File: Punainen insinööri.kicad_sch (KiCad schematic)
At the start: 28 parts, among them J1 Barrel_Jack_Switch, Q1 MMBF4393LT1G, SW1 SW_DPDT_x2, U1 LF351D

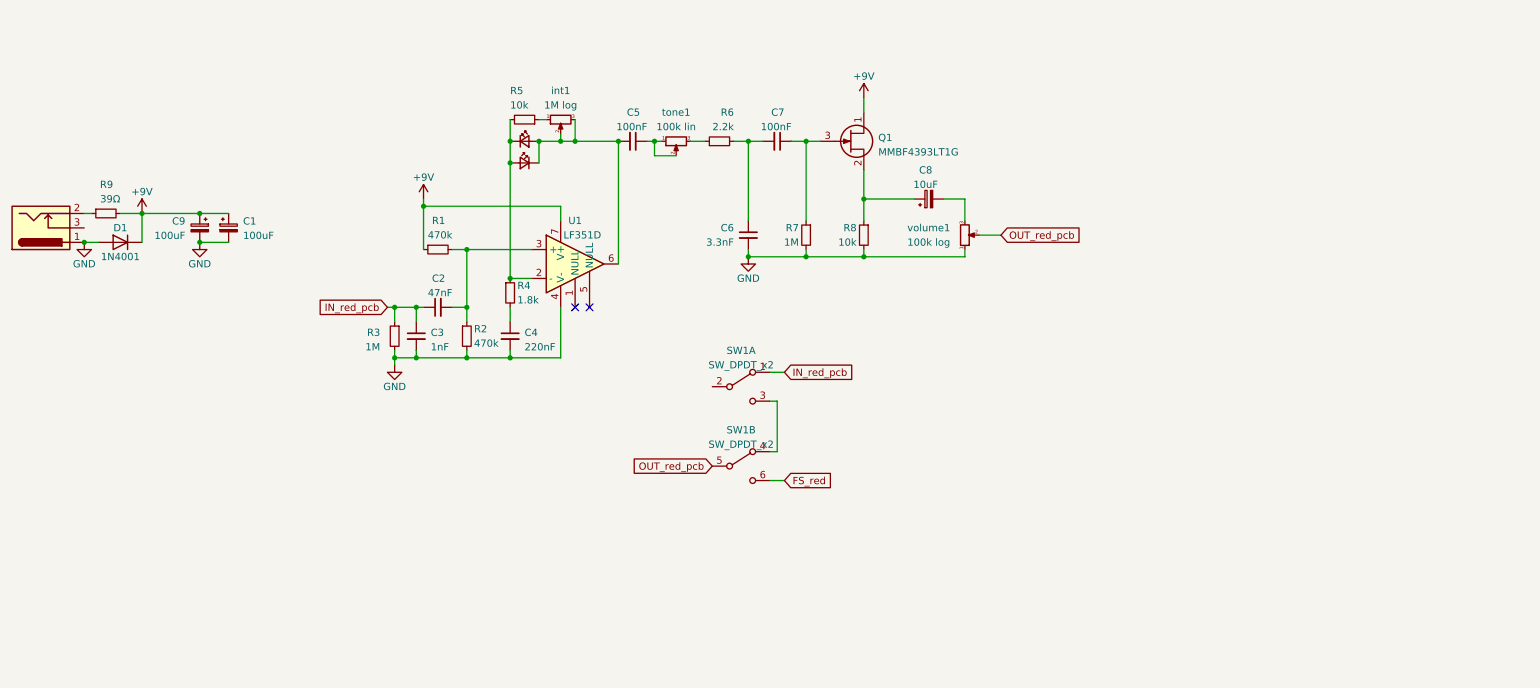
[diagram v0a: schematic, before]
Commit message: small fixes
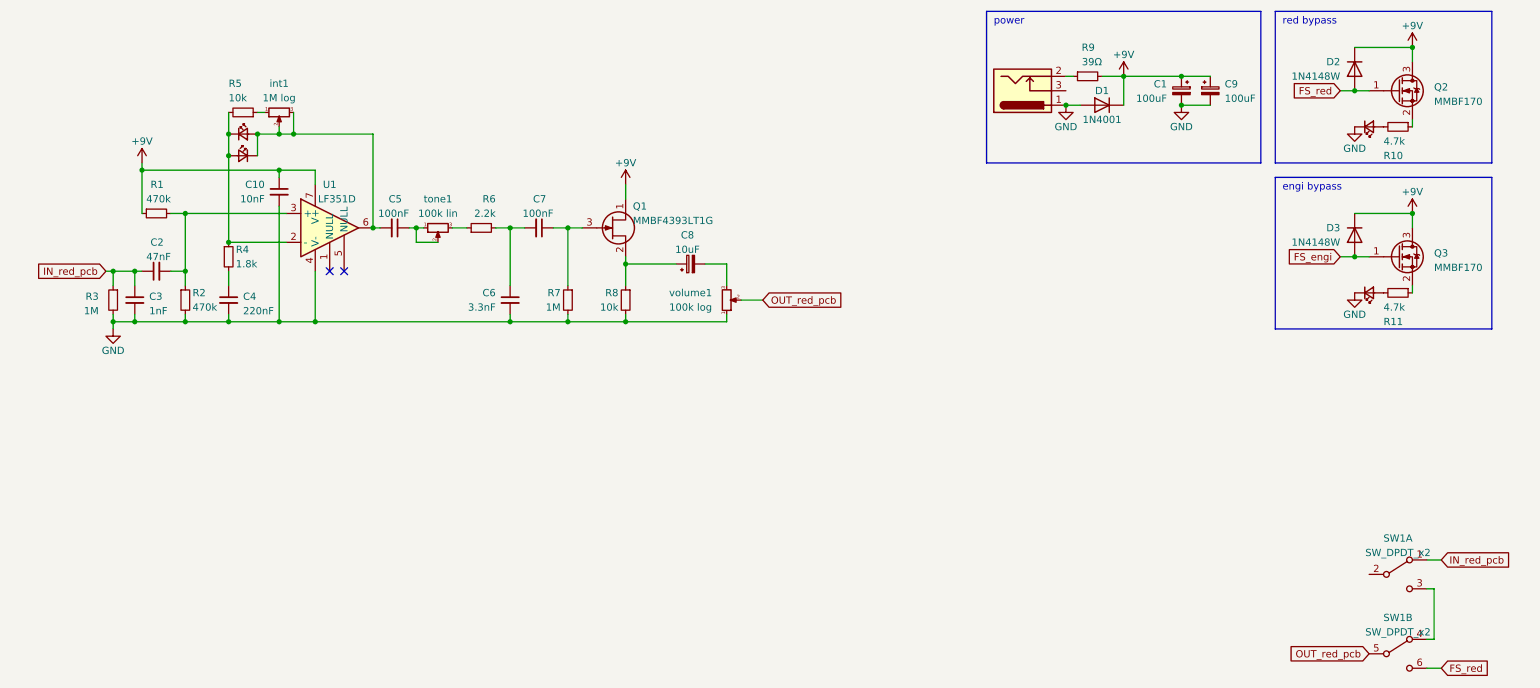
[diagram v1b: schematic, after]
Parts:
- added C10: 10nF, Capacitor_SMD:C_0805_2012Metric_Pad1.18x1.45mm_HandSolder, symbol Device:C_Small
- added D2, D3: 1N4148W, Diode_SMD:D_SOD-123, symbol Diode:1N4148W
- added LED3, LED4: LED_Small, symbol Device:LED_Small
- added Q2, Q3: MMBF170, Package_TO_SOT_SMD:SOT-23, symbol Transistor_FET:MMBF170
- added R10, R11: 4.7k, Resistor_SMD:R_0805_2012Metric_Pad1.20x1.40mm_HandSolder, symbol Device:R_Small
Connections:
- net +9V: now also C10.1, D2.1 (K), D3.1 (K), Q2.3 (D), Q3.3 (D)
- net FS_red: now also D2.2 (A), Q2.1 (G)
- net GND: now also C10.2, LED3.1 (K), LED4.1 (K)
- new net: LED3.2 (A), R10.2
- new net: LED4.2 (A), R11.2
- new net: Q3.2 (S), R11.1
- new net: Q2.2 (S), R10.1
- new net FS_engi: D3.2 (A), Q3.1 (G)
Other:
- note added: "engi bypass"
- note added: "power"
- note added: "red bypass"
- moved on the sheet: C2, C3, C4, C5, C6, C7, C8, Q1, R1, R2, R3, R4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

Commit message: millenials in shambles
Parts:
- LED1, LED2: footprint (none) -> LED_SMD:LED_1206_3216Metric_Pad1.42x1.75mm_HandSolder
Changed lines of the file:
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@@
       (effects (font (size 1.27 1.27)) hide)
     )
-    (property "Footprint" "" (at 59.69 36.83 90)
-      (effects (font (size 1.27 1.27)) hide)
-    )
-    (property "Datasheet" "~" (at 59.69 36.83 90)
+    (property "Footprint" "LED_SMD:LED_1206_3216Metric_Pad1.42x1.75mm_HandSolder" (at 59.69 36.83 90)
+      (effects (font (size 1.27 1.27)) hide)
+    )
+    (property "Datasheet" "C2827254" (at 59.69 36.83 90)
       (effects (font (size 1.27 1.27)) hide)
     )
@@
       (effects (font (size 1.27 1.27)) hide)
     )
-    (property "Footprint" "" (at 59.69 40.64 90)
-      (effects (font (size 1.27 1.27)) hide)
-    )
-    (property "Datasheet" "~" (at 59.69 40.64 90)
-      (effects (font (size 1.27 1.27)) hide)
-    )
+    (property "Footprint" "LED_SMD:LED_1206_3216Metric_Pad1.42x1.75mm_HandSolder" (at 59.69 40.64 90)
+      (effects (font (size 1.27 1.27)) hide)
+    )
+    (property "Datasheet" "C2827254" (at 59.69 40.64 90)
+      (effects (font (size 1.27 1.27)) hide)
+    )
